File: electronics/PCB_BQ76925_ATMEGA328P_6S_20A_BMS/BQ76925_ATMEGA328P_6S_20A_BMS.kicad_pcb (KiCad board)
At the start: 2 copper layers, 47 x 90 mm, 79 parts, among them J1 Conn_01x01, J2 Conn_01x01, J3 Conn_01x09, J4 Conn_01x02, J5 Conn_02x03, J6 Conn_01x04, Q1 BC817, Q2 IRFB4110, Q3 IRFB4110, Q4 IRFB4110, Q5 IRFB4110, U1 BQ76925PW, U2 LMR50410, U3 ATmega328P-A, U4 AMS1117-5.0, Y1 16Mhz

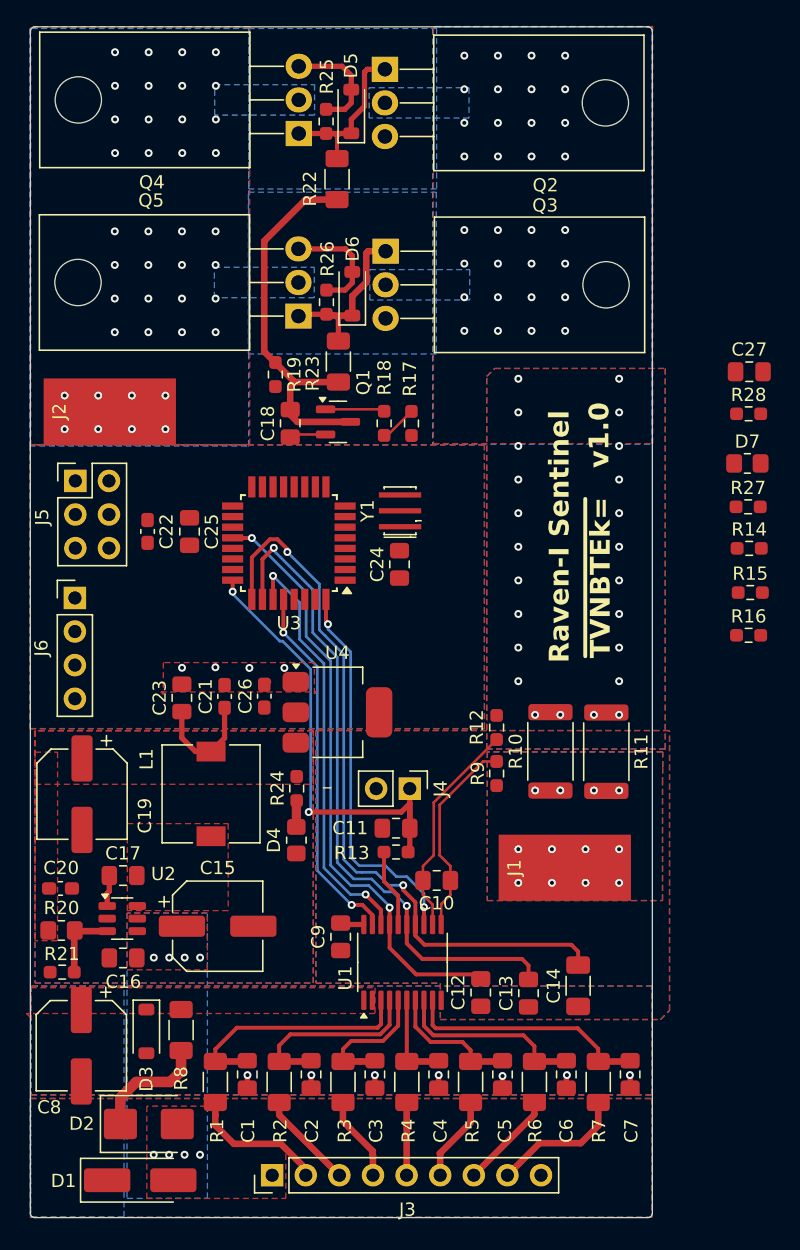
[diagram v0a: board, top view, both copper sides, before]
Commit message: pcb placement and 90 percent routed
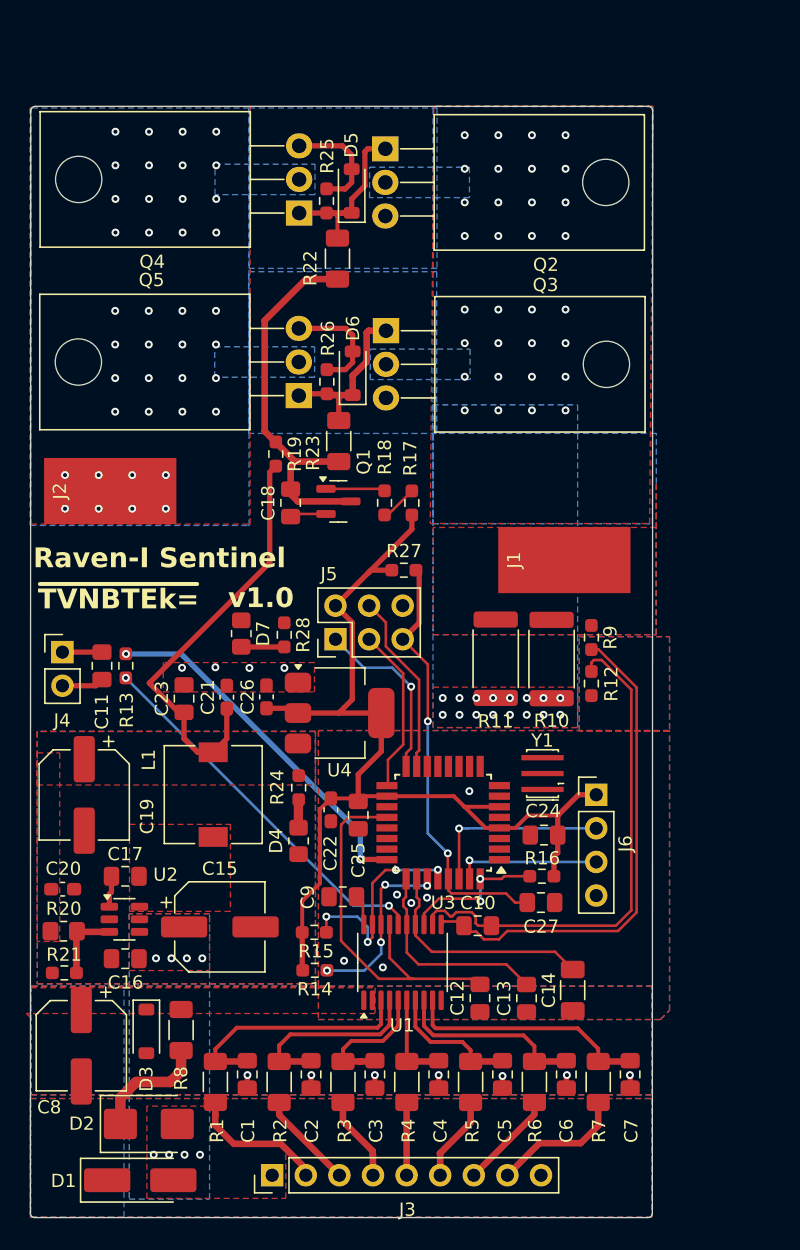
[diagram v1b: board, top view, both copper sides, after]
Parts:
- moved R14 45.8 mm to (137.0, 120.9), turned to 180 degrees
- moved C27 43.1 mm to (154.1, 115.8)
- moved J6 42.1 mm to (158.3, 107.6)
- moved R15 41.8 mm to (137.0, 118.0), turned to 180 degrees
- moved D7 40.4 mm to (131.5, 95.5), turned to -90 degrees
- moved R28 38.9 mm to (134.7, 95.6), turned to -90 degrees
- moved J4 28.2 mm to (117.9, 96.9), turned to 0 degrees
- moved R27 26.5 mm to (143.8, 90.7), turned to 180 degrees
- moved C11 25.4 mm to (120.9, 97.9), turned to 90 degrees
- moved C22 25.2 mm to (138.2, 108.8)
- moved C25 24.9 mm to (140.3, 109.2)
- moved R13 24.8 mm to (122.7, 97.9), turned to -90 degrees
- moved U3 24.1 mm to (146.7, 109.8)
- moved R16 24.0 mm to (154.2, 113.8)
- moved J1 23.3 mm to (155.9, 89.9)
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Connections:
- J5 pad 2: /MCU/SCK -> +5V
- J5 pad 3: /MCU/~{RESET} -> /MCU/SCK
- J5 pad 4: GND -> /MCU/MOSI
- J5 pad 5: /MCU/MOSI -> /MCU/~{RESET}
- J5 pad 6: +5V -> GND
- U3 pad 25: /24V 6 Cell Monitoring/VIOUT -> /24V 6 Cell Monitoring/VCOUT
- U3 pad 26: /24V 6 Cell Monitoring/VCOUT -> /24V 6 Cell Monitoring/VIOUT
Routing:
- net +5V: track 0.00 -> 80.0 mm
- net /24V 6 Cell Monitoring/VIOUT: track 55.3 -> 17.4 mm, vias 2 -> 0
- net /24V 6 Cell Monitoring/VCOUT: track 50.5 -> 15.8 mm, vias 2 -> 0
- net /MCU/~{RESET}: track 0.00 -> 32.6 mm, vias 0 -> 2
- net +12V: track 8.35 -> 32.2 mm
- net Net-(U1-VTB): track 5.92 -> 28.7 mm, vias 0 -> 2
- net /24V 6 Cell Monitoring/A+: track 15.3 -> 37.9 mm
- net /24V 6 Cell Monitoring/A-: track 16.6 -> 38.8 mm
- net /24V 6 Cell Monitoring/SDA: track 32.2 -> 13.2 mm, vias 2 -> 4
- net /24V 6 Cell Monitoring/ALERT: track 29.3 -> 11.2 mm
- net /24V 6 Cell Monitoring/VREF: track 45.4 -> 29.3 mm, vias 2 -> 0
- net /MCU/RXD: track 0.00 -> 14.2 mm, vias 0 -> 1
- net /MCU/MOSI: track 0.00 -> 13.8 mm
- net /MCU/MISO: track 0.00 -> 13.4 mm, vias 0 -> 1
- net /MCU/SCK: track 0.00 -> 12.6 mm
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- removed copper zone on F.Cu, net +5V
- removed copper zone on B.Cu, net /24V 6 Cell Monitoring/BAT-
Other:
- board size 47 x 90 mm -> 47 x 84 mm
